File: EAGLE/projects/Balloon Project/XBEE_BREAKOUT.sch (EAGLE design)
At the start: 2 parts

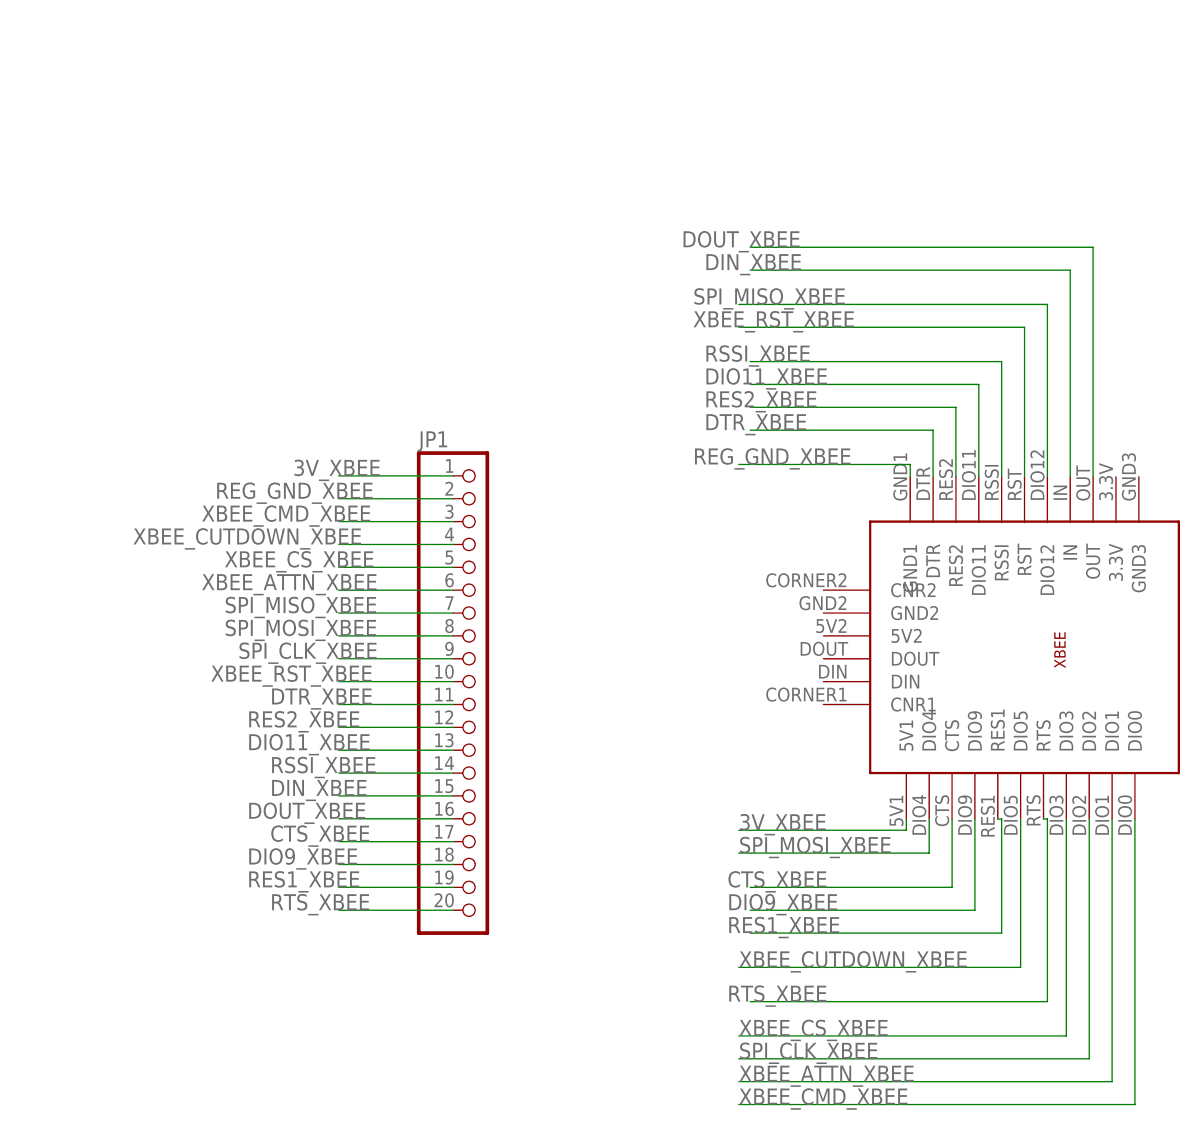
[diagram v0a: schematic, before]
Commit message: gerber files generated
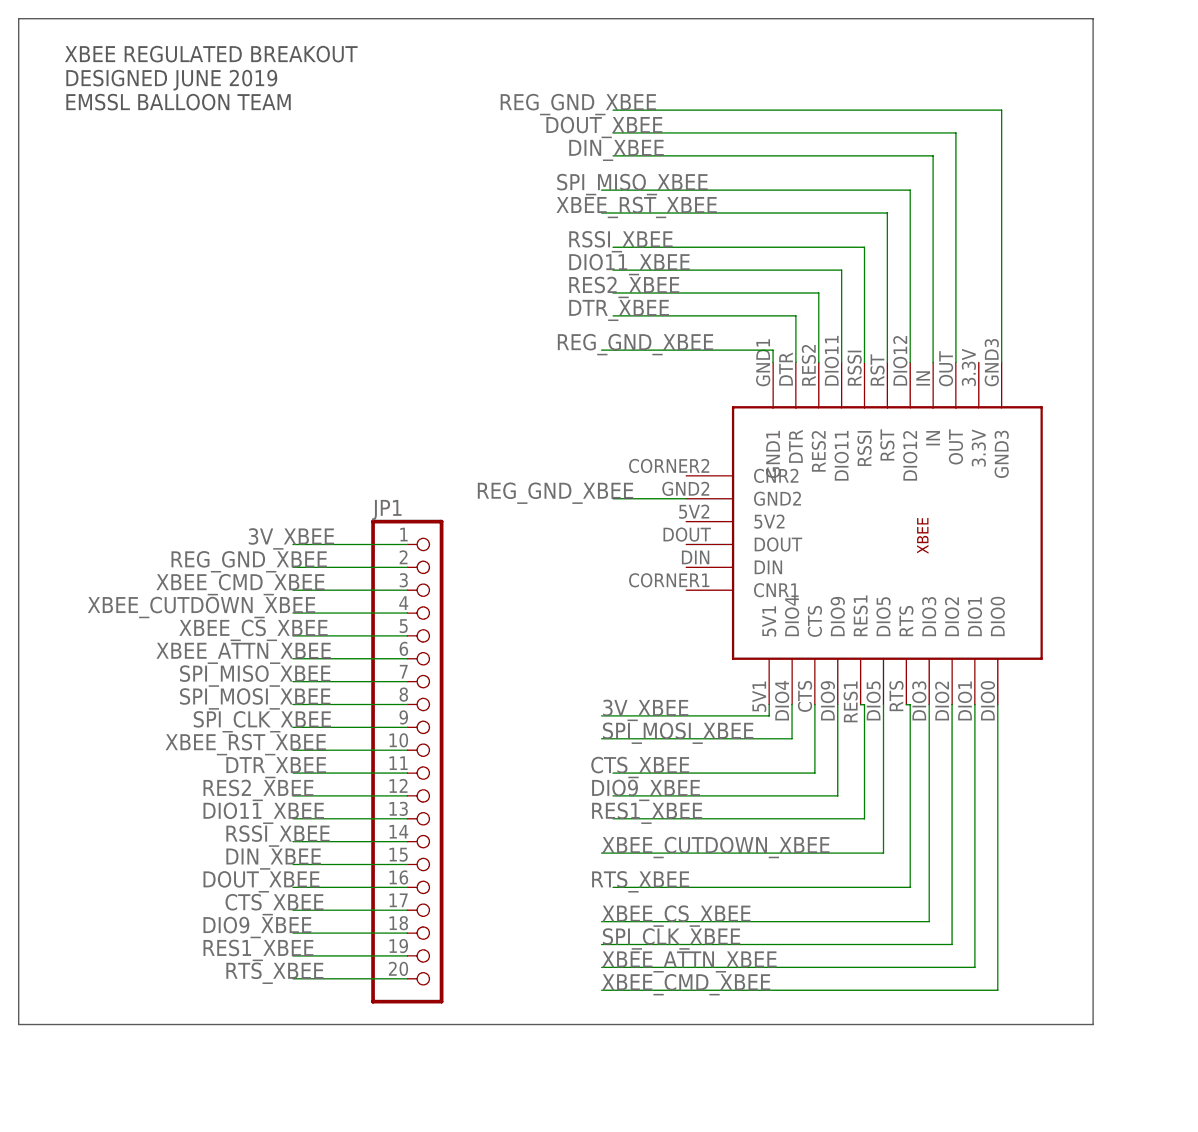
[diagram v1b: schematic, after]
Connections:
- net REG_GND_XBEE: now also U$7.GND2, U$7.GND3
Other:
- note added: "XBEE REGULATED BREAKOUT DESIGNED JUNE 2019 EMSSL BALLOON TEAM"
- moved on the sheet: JP1
